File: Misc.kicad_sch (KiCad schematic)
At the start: 22 parts, among them J2 TE 338069-4, J3 Conn_02x08_Odd_Even, J4 BM04B-SURS-TFLFSN, J5 Conn_02x04_Odd_Even, J6 Conn_02x04_Odd_Even, J7 Conn_01x05, U5 SN65HVD232QDRQ1

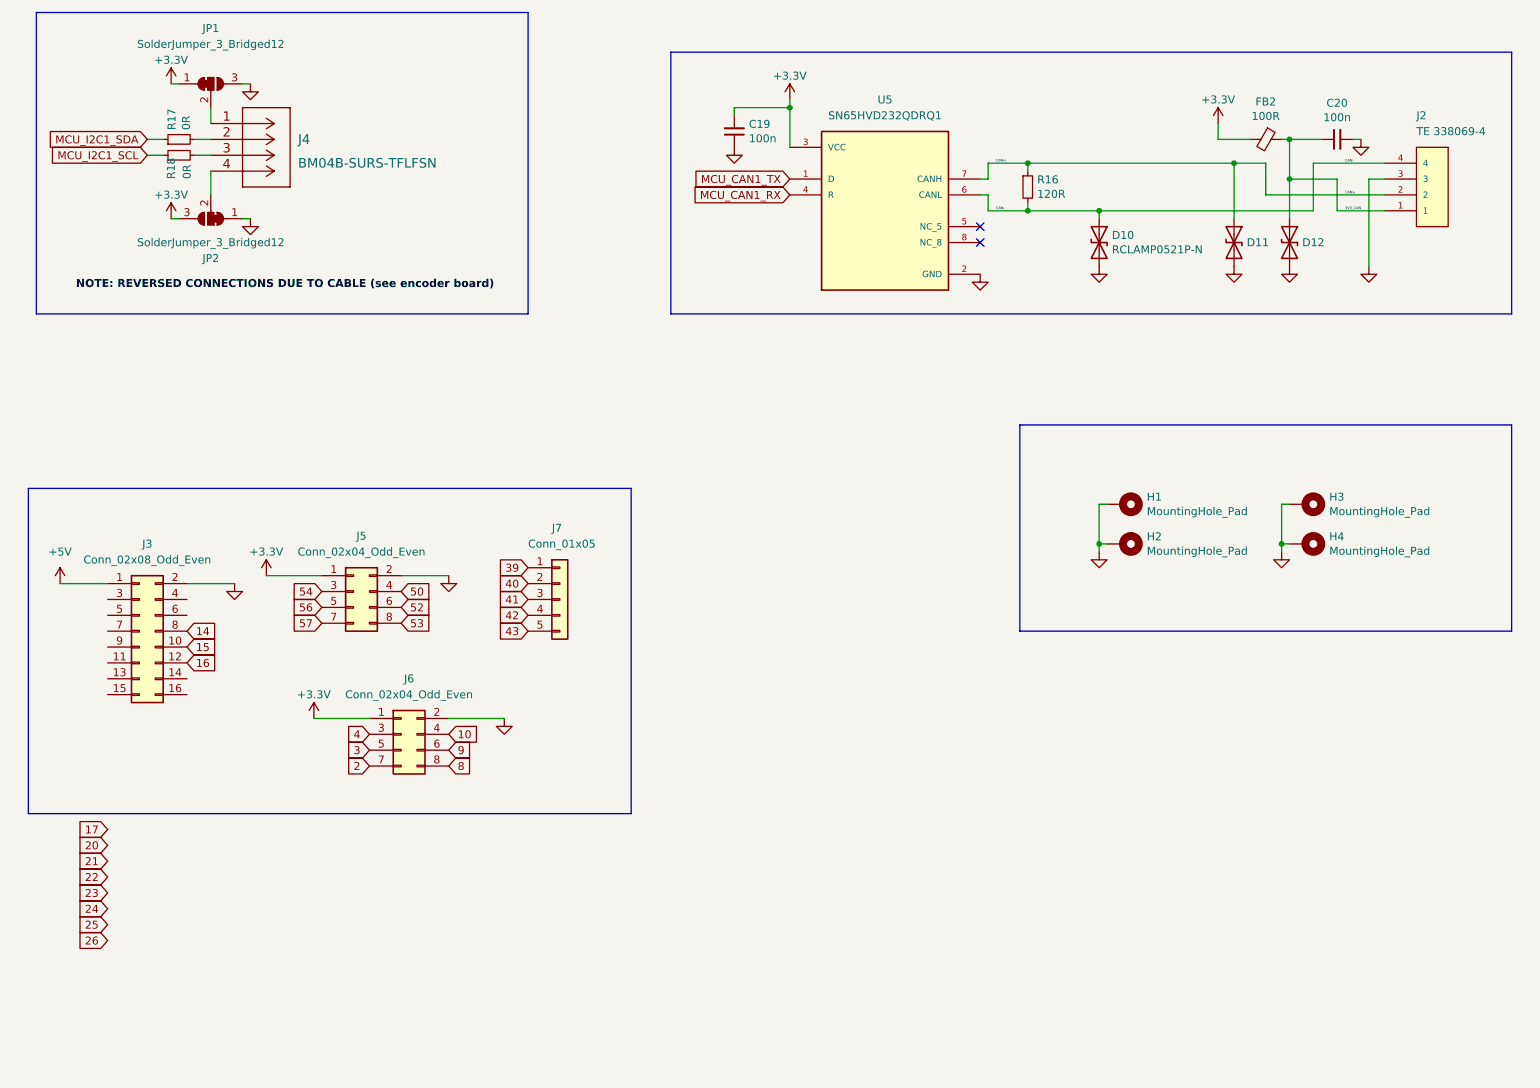
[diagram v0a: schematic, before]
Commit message: adsigjningh
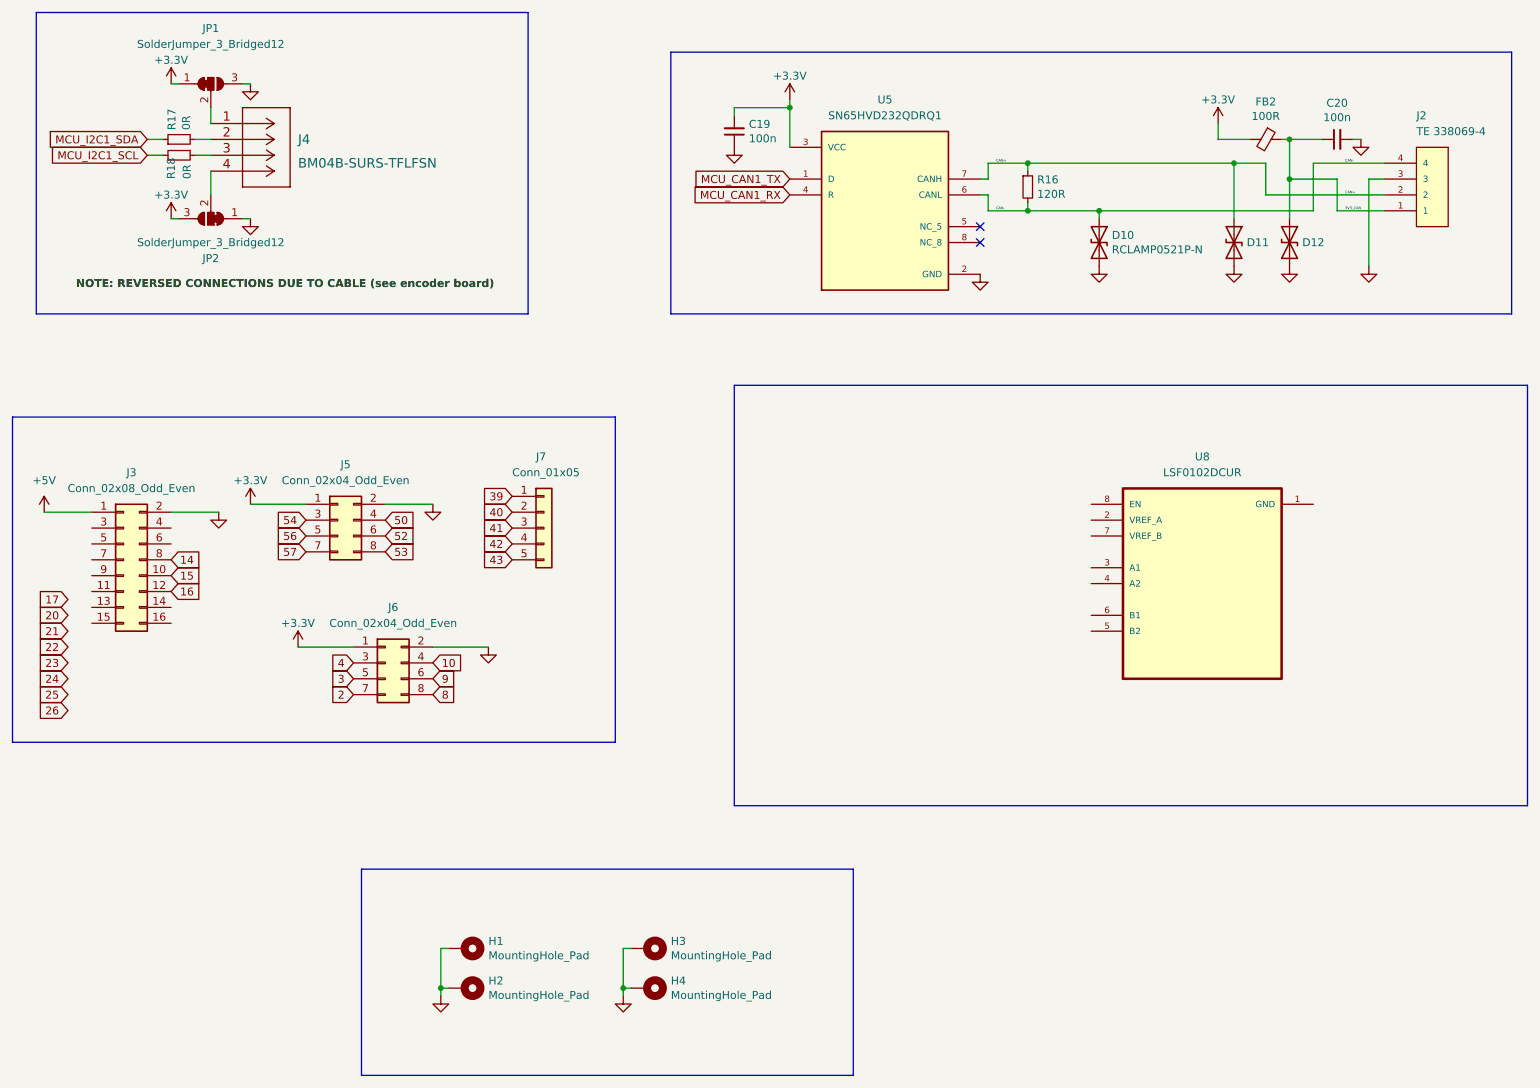
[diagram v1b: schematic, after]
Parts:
- added U8: LSF0102DCUR, SnapEDA Library:SOP50P310X90-8N, symbol LSF0102DCUR:LSF0102DCUR
- J4: footprint BM04B:BM04B-SURS-TFLFSN -> SnapEDA Library:JST_BM04B-SURS-TF(LF)(SN)
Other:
- moved on the sheet: H1, H2, H3, H4, J3, J5, J6, J7
